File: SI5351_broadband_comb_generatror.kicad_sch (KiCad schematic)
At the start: 4 parts, among them J1 Conn_Coaxial_Small, J3 Barrel_Jack_Switch, J4 Conn_Coaxial_Small, J9 Conn_Coaxial_Small

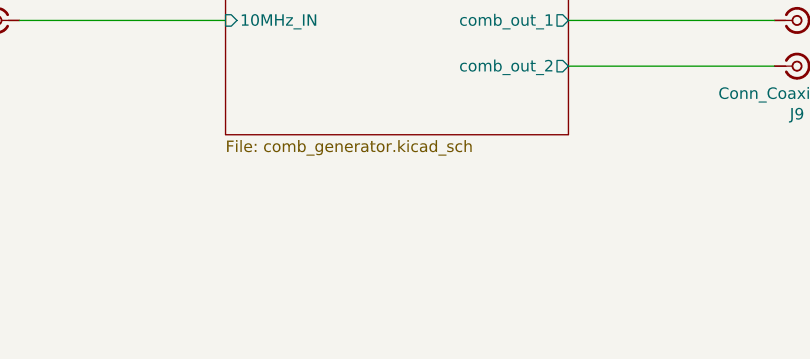
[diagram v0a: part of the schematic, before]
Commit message: es wird langsam...
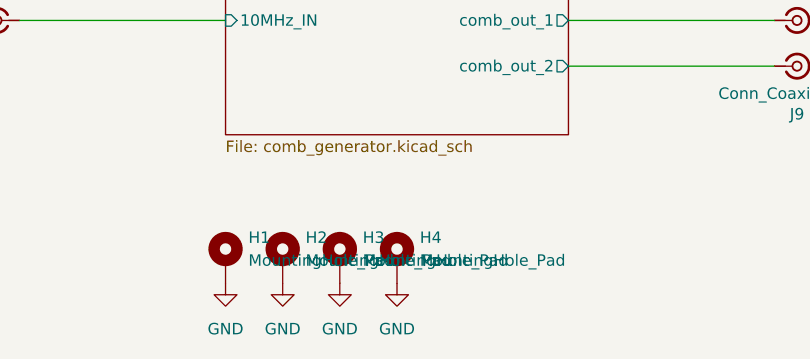
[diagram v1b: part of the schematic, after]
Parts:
- added H1, H2, H3, H4: MountingHole_Pad, MountingHole:MountingHole_3.2mm_M3_Pad_Via, symbol Mechanical:MountingHole_Pad
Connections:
- net GND: now also H1.1, H2.1, H3.1, H4.1

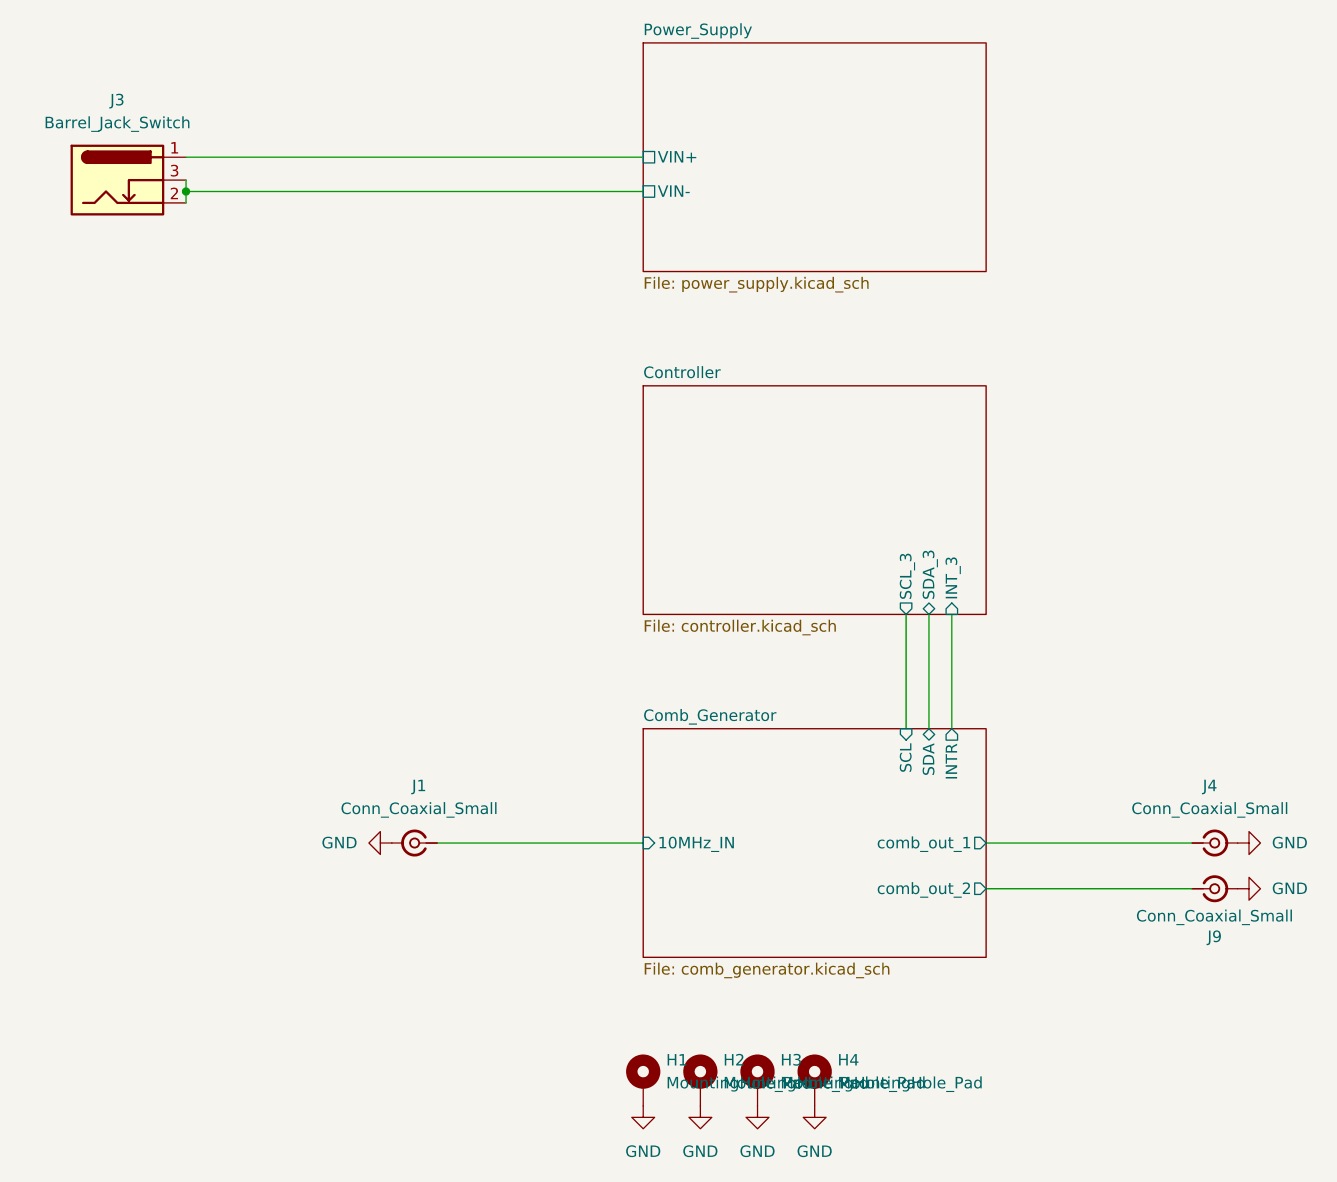
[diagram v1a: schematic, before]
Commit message: BOM angefangen und im Layout vom Hundertsten ins Tausendste gekommen...
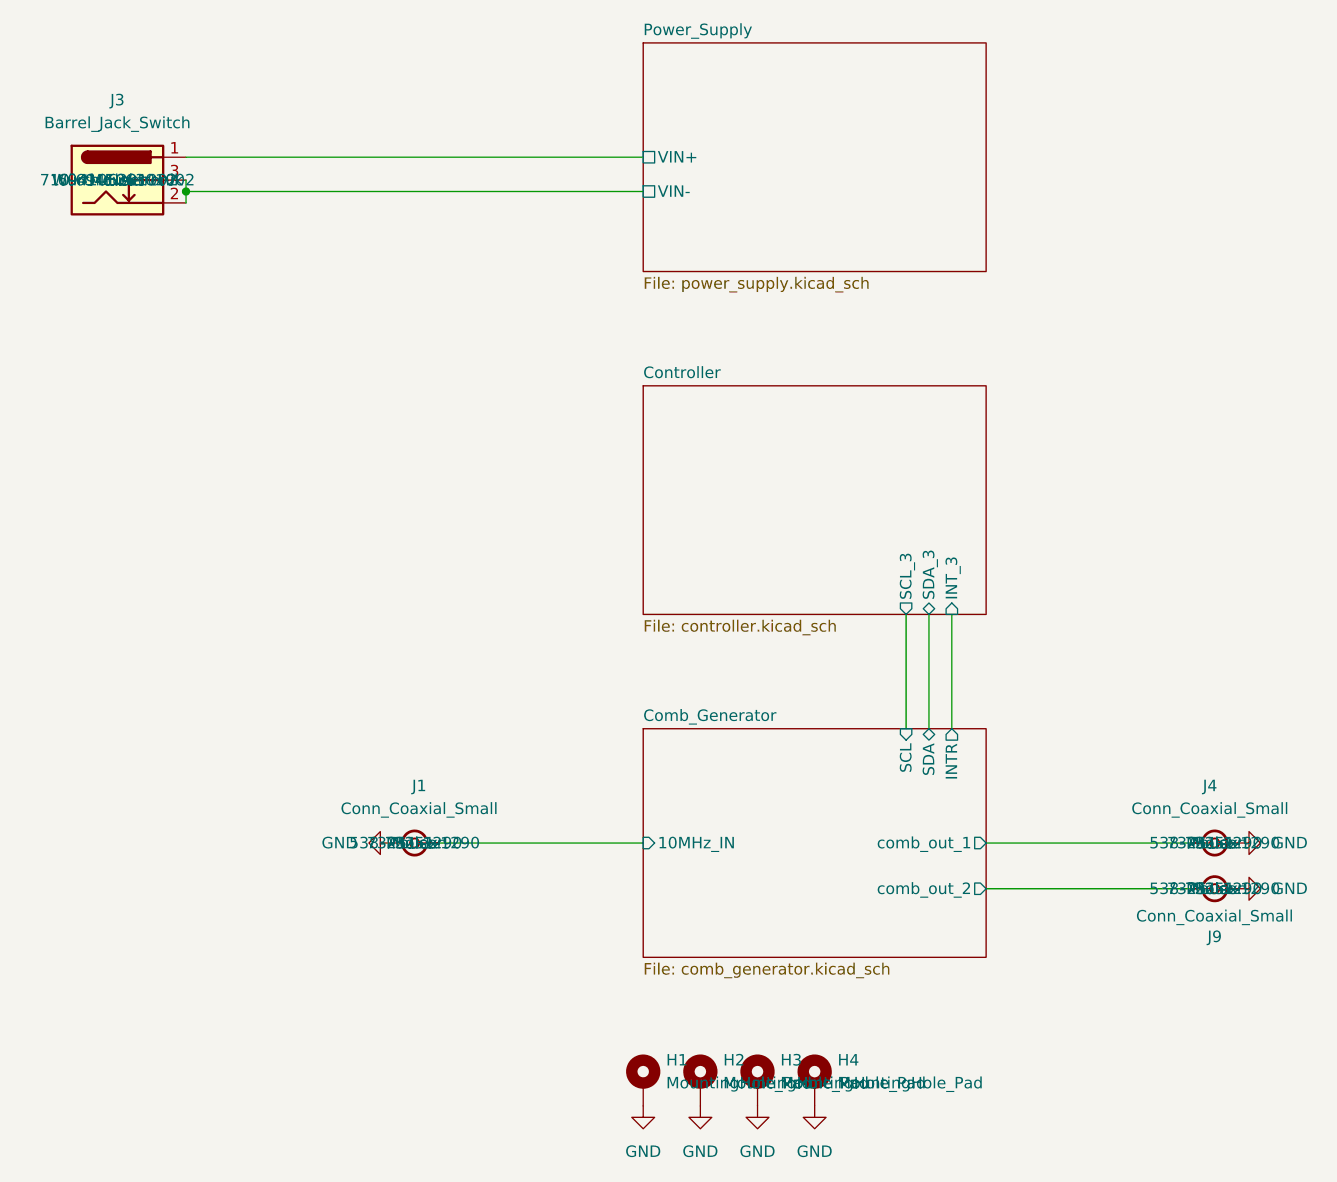
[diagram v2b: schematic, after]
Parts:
- J1, J4, J9: Distributor (none) -> Mouser; Distributor PN (none) -> 538-73251-1290; Manufacturer (none) -> Molex; Manufacturer PN (none) -> 73251-1290
- J3: Distributor (none) -> Mouser; Distributor PN (none) -> 710-694106301002; Manufacturer (none) -> Würth Elektronik; Manufacturer PN (none) -> 694106301002
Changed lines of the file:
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@@
+			)
+		)
+		(property "Distributor" "Mouser"
+			(at 101.6 127 0)
+			(effects
+				(font
+					(size 1.27 1.27)
+				)
+			)
+		)
+		(property "Distributor PN" " 538-73251-1290"
+			(at 101.6 127 0)
+			(effects
+				(font
+					(size 1.27 1.27)
+				)
+			)
+		)
+		(property "Manufacturer" "Molex "
+			(at 101.6 127 0)
+			(effects
+				(font
+					(size 1.27 1.27)
+				)
+			)
+		)
+		(property "Manufacturer PN" "73251-1290"
+			(at 101.6 127 0)
+			(effects
+				(font
+					(size 1.27 1.27)
+				)
 			)
 		)
@@
 			)
 		)
+		(property "Distributor" "Mouser"
+			(at 190.5 127 0)
+			(effects
+				(font
+					(size 1.27 1.27)
+				)
+			)
+		)
+		(property "Distributor PN" " 538-73251-1290"
+			(at 190.5 127 0)
+			(effects
+				(font
+					(size 1.27 1.27)
+				)
+			)
+		)
+		(property "Manufacturer" "Molex "
+			(at 190.5 127 0)
+			(effects
+				(font
+					(size 1.27 1.27)
+				)
+			)
+		)
+		(property "Manufacturer PN" "73251-1290"
+			(at 190.5 127 0)
+			(effects
+				(font
+					(size 1.27 1.27)
+				)
+			)
+		)
 		(pin "1"
 		)
@@
 			)
 		)
+		(property "Distributor" "Mouser"
+			(at 68.58 53.34 0)
+			(effects
+				(font
+					(size 1.27 1.27)
+				)
+			)
+		)
+		(property "Distributor PN" " 710-694106301002 "
+			(at 68.58 53.34 0)
+			(effects
+				(font
+					(size 1.27 1.27)
+				)
+			)
+		)
+		(property "Manufacturer" "Würth Elektronik"
+			(at 68.58 53.34 0)
+			(effects
+				(font
+					(size 1.27 1.27)
+				)
+			)
+		)
+		(property "Manufacturer PN" "694106301002"
+			(at 68.58 53.34 0)
+			(effects
+				(font
+					(size 1.27 1.27)
+				)
+			)
+		)
 		(pin "1"
 		)
@@
 			)
 		)
+		(property "Distributor" "Mouser"
+			(at 190.5 132.08 0)
+			(effects
+				(font
+					(size 1.27 1.27)
+				)
+			)
+		)
+		(property "Distributor PN" " 538-73251-1290"
+			(at 190.5 132.08 0)
+			(effects
+				(font
+					(size 1.27 1.27)
+				)
+			)
+		)
+		(property "Manufacturer" "Molex "
+			(at 190.5 132.08 0)
+			(effects
+				(font
+					(size 1.27 1.27)
+				)
+			)
+		)
+		(property "Manufacturer PN" "73251-1290"
+			(at 190.5 132.08 0)
+			(effects
+				(font
+					(size 1.27 1.27)
+				)
+			)
+		)
